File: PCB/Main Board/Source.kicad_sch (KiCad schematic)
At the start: 45 parts, among them K1 G2RL-1, U1 OPA1662

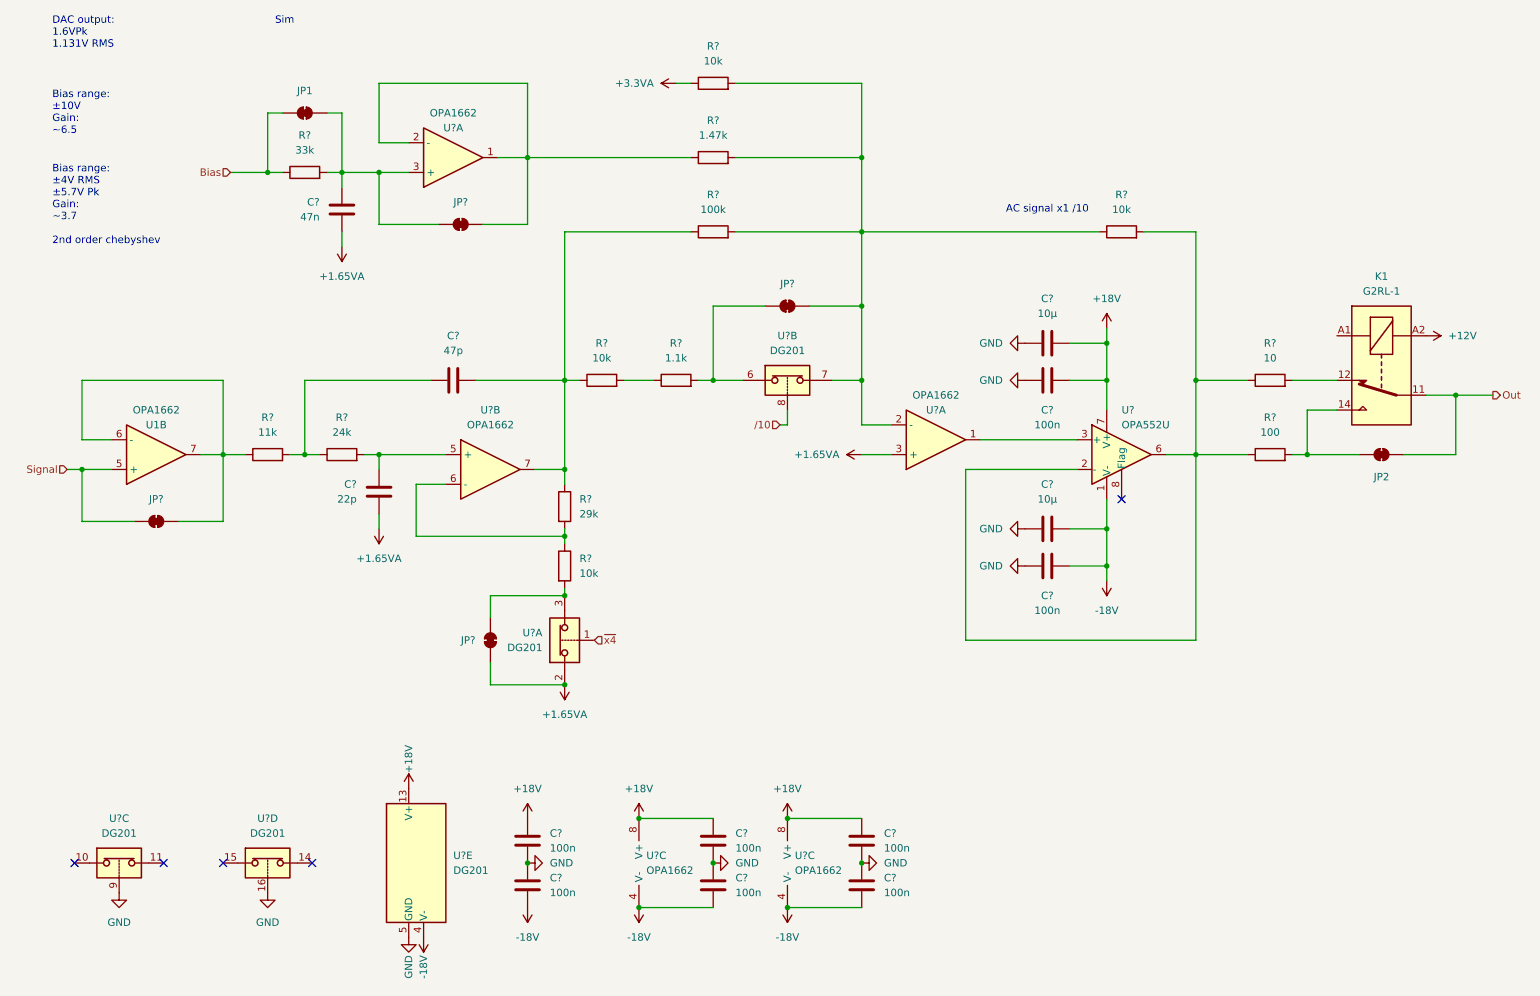
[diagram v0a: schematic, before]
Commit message: Amplifier Switch
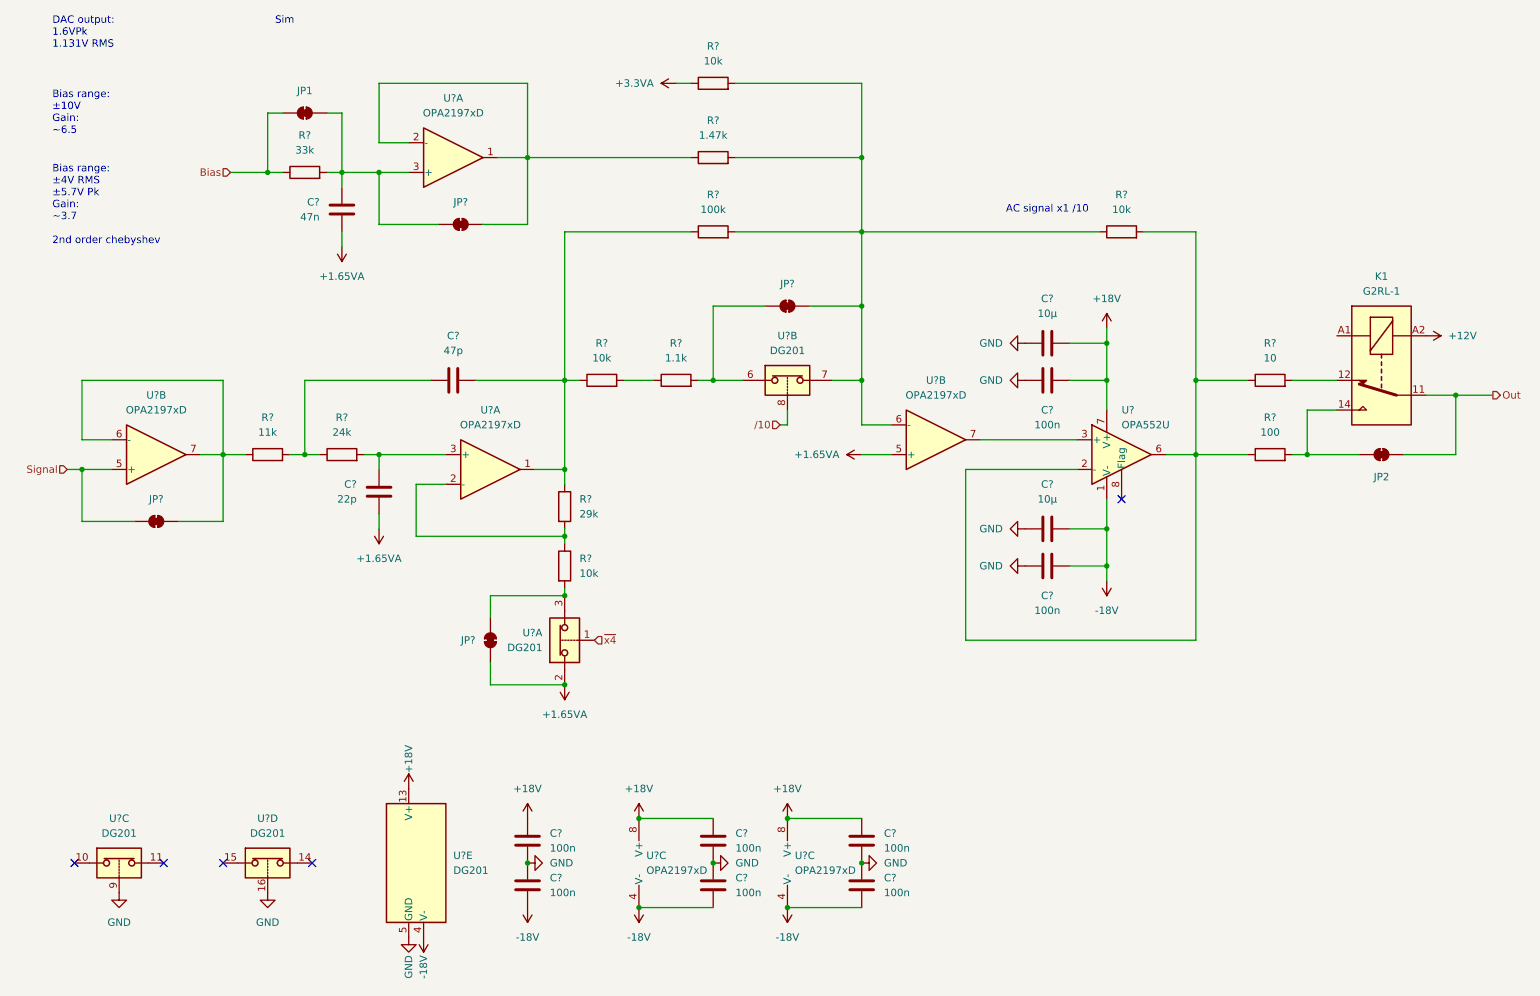
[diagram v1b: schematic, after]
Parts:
- removed U1, U? (x5): OPA1662, Package_SO:SOIC-8_3.9x4.9mm_P1.27mm, symbol Device:Opamp_Dual
- added U? (x6): OPA2197xD, Package_SO:SOIC-8_3.9x4.9mm_P1.27mm, symbol Amplifier_Operational:OPA2197xD
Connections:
- net +1.65VA: now also U?.5 (+)
- net +18V: now also U?.8 (V+), U?.8 (V+)
- net -18V: now also U?.4 (V-), U?.4 (V-)
- net Signal: now also U?.5 (+)
- net at C?.2, R?.1, R?.1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: now also U?.1
- net at C?.1, R?.2: now also U?.3 (+)
- net at R?.1, R?.2: now also U?.2 (-)
- net at JP?.2 (B), R?.1, R?.2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: now also U?.6 (-)
- net at JP?.2 (B), R?.1: now also U?.6 (-), U?.7
- net at JP?.2 (B), R?.1: now also U?.1, U?.2 (-)
- net at C?.1, JP1.2 (B), JP?.1 (A)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: now also U?.3 (+)
- net at U?.3 (+): now also U?.7
